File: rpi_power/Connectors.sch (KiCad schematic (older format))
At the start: 6 parts, among them J1 POWER, J2 Raspberry_Pi_2_3, J3 Raspberry_Pi_2_3, J4 ADCs, J7 PROG, J9 GPIO

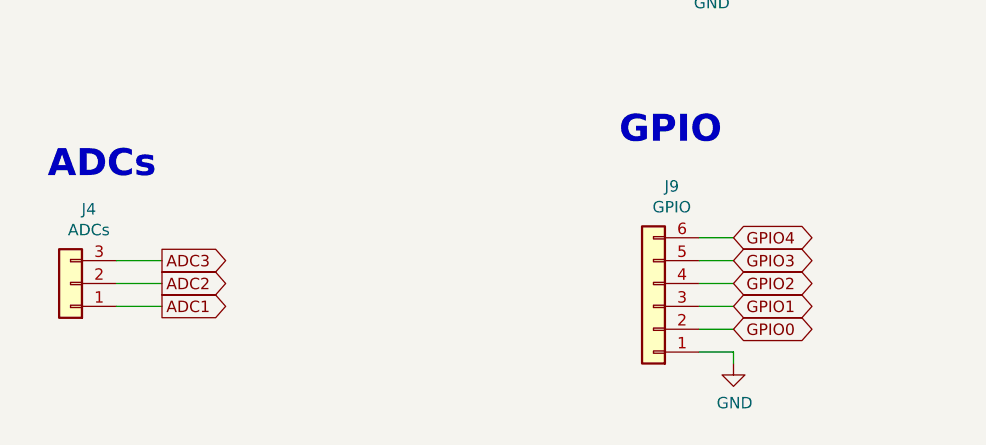
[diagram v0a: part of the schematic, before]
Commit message: Components placed.
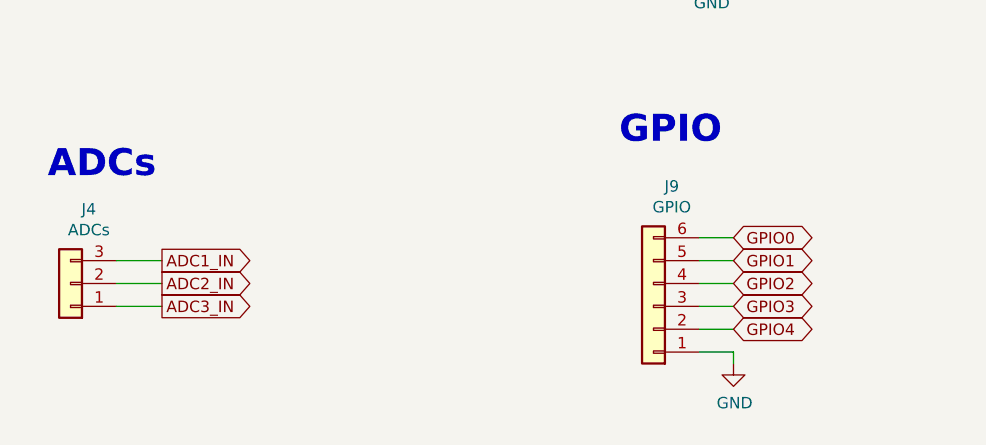
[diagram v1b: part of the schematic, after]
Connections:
- net GPIO0: now also J9.6 (Pin_6); no longer J9.2 (Pin_2)
- net GPIO1: now also J9.5 (Pin_5); no longer J9.3 (Pin_3)
- net GPIO3: now also J9.3 (Pin_3); no longer J9.5 (Pin_5)
- net GPIO4: now also J9.2 (Pin_2); no longer J9.6 (Pin_6)
- net ADC1 renamed ADC3_IN
- net ADC2 renamed ADC2_IN
- net ADC3 renamed ADC1_IN
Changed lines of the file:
@@
 Wire Wire Line
 	4950 5750 5150 5750
+Text GLabel 5150 5550 2    50   Output ~ 0
+ADC1_IN
+Text GLabel 5150 5650 2    50   Output ~ 0
+ADC2_IN
 Text GLabel 5150 5750 2    50   Output ~ 0
-ADC1
-Text GLabel 5150 5650 2    50   Output ~ 0
-ADC2
-Text GLabel 5150 5550 2    50   Output ~ 0
-ADC3
+ADC3_IN
 $Comp
 L Connector:Conn_01x06_Male J?
@@
 Wire Wire Line
 	7500 5450 7650 5450
-Text GLabel 7650 5850 2    50   BiDi ~ 0
+Text GLabel 7650 5450 2    50   BiDi ~ 0
 GPIO0
 $Comp
@@
 	-1   0    0    1
 $EndComp
-Text GLabel 7650 5750 2    50   BiDi ~ 0
+Text GLabel 7650 5550 2    50   BiDi ~ 0
 GPIO1
 Text GLabel 7650 5650 2    50   BiDi ~ 0
 GPIO2
-Text GLabel 7650 5550 2    50   BiDi ~ 0
+Text GLabel 7650 5750 2    50   BiDi ~ 0
 GPIO3
-Text GLabel 7650 5450 2    50   BiDi ~ 0
+Text GLabel 7650 5850 2    50   BiDi ~ 0
 GPIO4
 Text GLabel 4100 1750 2    50   UnSpc ~ 0

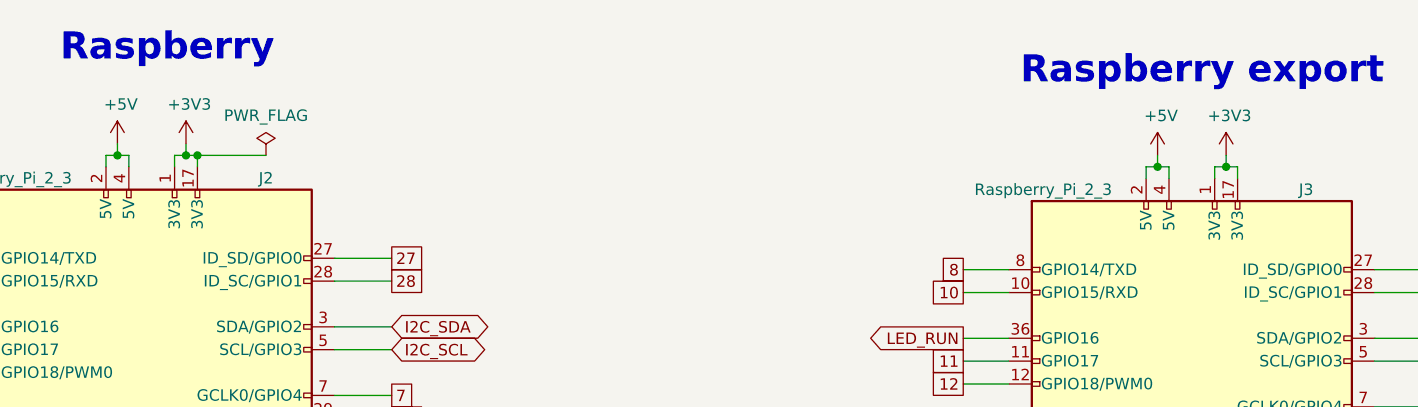
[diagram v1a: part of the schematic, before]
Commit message: Routing done, pending review.
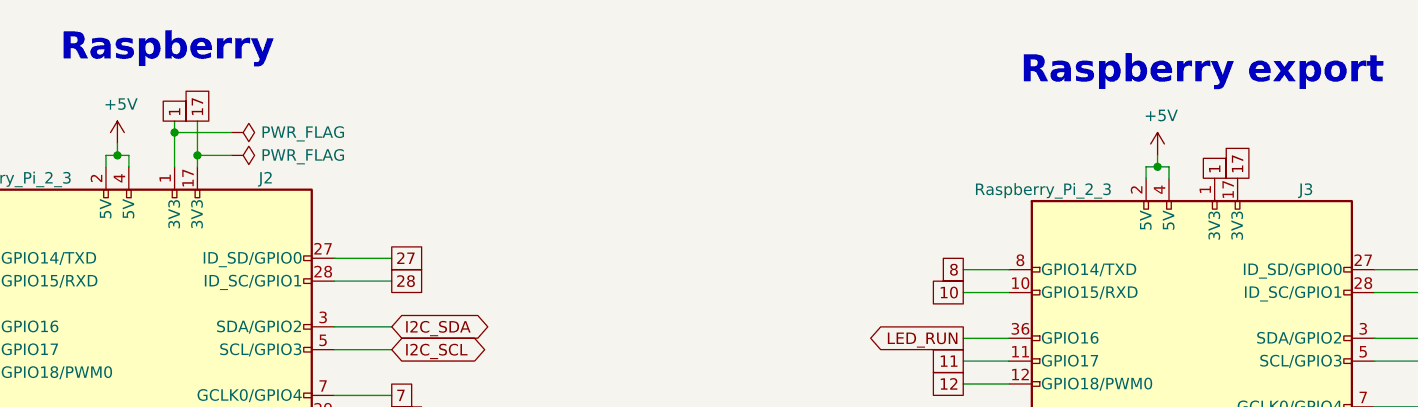
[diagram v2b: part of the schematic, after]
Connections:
- net +3V3 renamed 1
- net 1: no longer J2.17 (3V3), J3.17 (3V3)
- new net 17: J2.17 (3V3), J3.17 (3V3)
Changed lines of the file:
@@
 	2850 1350 2850 1300
-Wire Wire Line
-	3150 1350 3150 1300
-Wire Wire Line
-	3250 1350 3250 1300
 Wire Wire Line
 	3850 1750 4100 1750
@@
 	2850 1300 2900 1300
 Wire Wire Line
-	3150 1300 3200 1300
-Wire Wire Line
 	2950 1300 2950 1350
 Wire Wire Line
@@
 Wire Wire Line
 	2900 1300 2950 1300
-Wire Wire Line
-	3200 1300 3200 1250
-Connection ~ 3200 1300
-Wire Wire Line
-	3200 1300 3250 1300
 $Comp
 L power:+5V #PWR03
@@
 F 3 "" H 2900 1250 50  0001 C CNN
 	1    2900 1250
-	1    0    0    -1
-$EndComp
-$Comp
-L power:+3V3 #PWR05
-U 1 1 5BE0BE90
-P 3200 1250
-F 0 "#PWR05" H 3200 1100 50  0001 C CNN
-F 1 "+3V3" H 3215 1423 50  0000 C CNN
-F 2 "" H 3200 1250 50  0001 C CNN
-F 3 "" H 3200 1250 50  0001 C CNN
-	1    3200 1250
 	1    0    0    -1
 $EndComp
@@
 Text GLabel 4100 2150 2    50   BiDi ~ 0
 I2C_SCL
-Wire Wire Line
-	3250 1300 3550 1300
-Connection ~ 3250 1300
-$Comp
-L power:PWR_FLAG #FLG03
-U 1 1 5BE8CB1B
-P 3550 1300
-F 0 "#FLG03" H 3550 1375 50  0001 C CNN
-F 1 "PWR_FLAG" H 3550 1474 50  0000 C CNN
-F 2 "" H 3550 1300 50  0001 C CNN
-F 3 "~" H 3550 1300 50  0001 C CNN
-	1    3550 1300
-	1    0    0    -1
-$EndComp
 $Comp
 L Connector_Generic:Conn_01x03 J1
@@
 	7400 1400 7400 1350
 Wire Wire Line
-	7700 1400 7700 1350
-Wire Wire Line
-	7800 1400 7800 1350
-Wire Wire Line
 	8400 1800 8650 1800
 Wire Wire Line
@@
 	7400 1350 7450 1350
 Wire Wire Line
-	7700 1350 7750 1350
-Wire Wire Line
 	7500 1350 7500 1400
 Wire Wire Line
@@
 Wire Wire Line
 	7450 1350 7500 1350
-Wire Wire Line
-	7750 1350 7750 1300
-Connection ~ 7750 1350
-Wire Wire Line
-	7750 1350 7800 1350
 $Comp
 L power:+5V #PWR014
@@
 F 3 "" H 7450 1300 50  0001 C CNN
 	1    7450 1300
-	1    0    0    -1
-$EndComp
-$Comp
-L power:+3V3 #PWR016
-U 1 1 5BEE7F48
-P 7750 1300
-F 0 "#PWR016" H 7750 1150 50  0001 C CNN
-F 1 "+3V3" H 7765 1473 50  0000 C CNN
-F 2 "" H 7750 1300 50  0001 C CNN
-F 3 "" H 7750 1300 50  0001 C CNN
-	1    7750 1300
 	1    0    0    -1
 $EndComp
@@
 Wire Wire Line
 	7650 5950 7650 6000
+Text GLabel 3150 1150 1    50   UnSpc ~ 0
+1
+Text GLabel 3250 1150 1    50   UnSpc ~ 0
+17
+Text GLabel 7700 1400 1    50   UnSpc ~ 0
+1
+Text GLabel 7800 1400 1    50   UnSpc ~ 0
+17
+Wire Wire Line
+	3150 1350 3150 1200
+Wire Wire Line
+	3250 1150 3250 1300
+$Comp
+L power:PWR_FLAG #FLG0101
+U 1 1 5BDC6759
+P 3400 1300
+F 0 "#FLG0101" H 3400 1375 50  0001 C CNN
+F 1 "PWR_FLAG" V 3400 1428 50  0000 L CNN
+F 2 "" H 3400 1300 50  0001 C CNN
+F 3 "~" H 3400 1300 50  0001 C CNN
+	1    3400 1300
+	0    1    1    0
+$EndComp
+Connection ~ 3250 1300
+Wire Wire Line
+	3250 1300 3250 1350
+$Comp
+L power:PWR_FLAG #FLG0102
+U 1 1 5BDC677F
+P 3400 1200
+F 0 "#FLG0102" H 3400 1275 50  0001 C CNN
+F 1 "PWR_FLAG" V 3400 1328 50  0000 L CNN
+F 2 "" H 3400 1200 50  0001 C CNN
+F 3 "~" H 3400 1200 50  0001 C CNN
+	1    3400 1200
+	0    1    1    0
+$EndComp
+Wire Wire Line
+	3250 1300 3400 1300
+Wire Wire Line
+	3400 1200 3150 1200
+Connection ~ 3150 1200
+Wire Wire Line
+	3150 1200 3150 1150
 $EndSCHEMATC
